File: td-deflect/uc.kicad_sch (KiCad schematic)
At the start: 20 parts, among them J4 Conn_ARM_JTAG_SWD_10, J6 Conn_01x06_Male, U12 LM1117-5.0, U2 STM32G474RETx, U23 TPS70933, U4 TPS70933, U8 INA181, X1 SG-8002CA

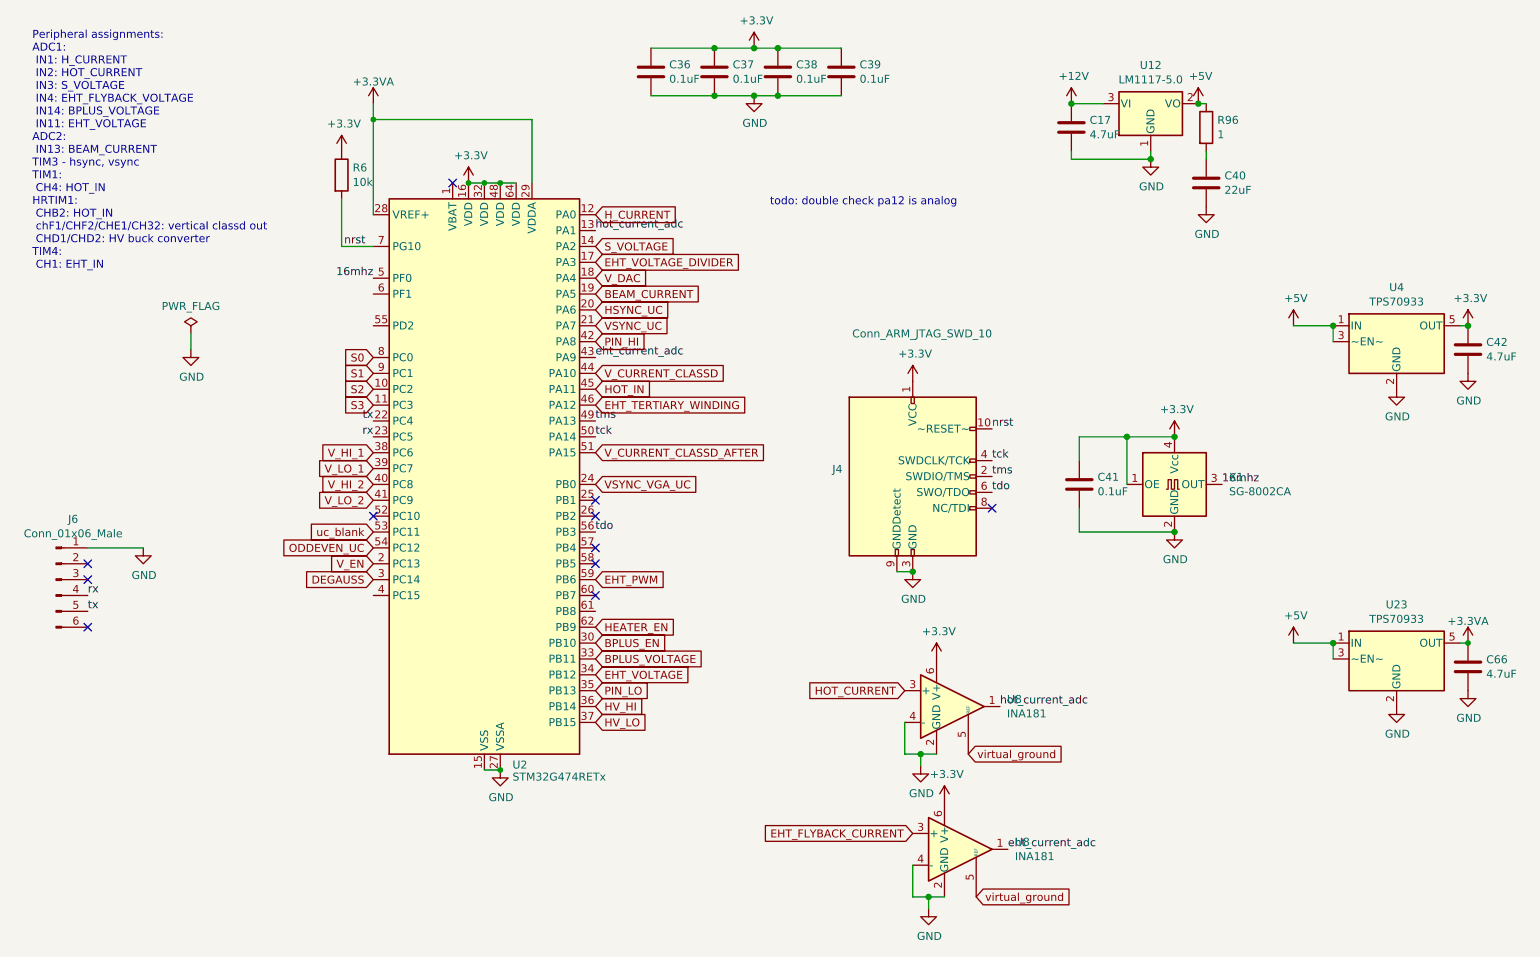
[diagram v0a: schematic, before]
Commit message: more updates
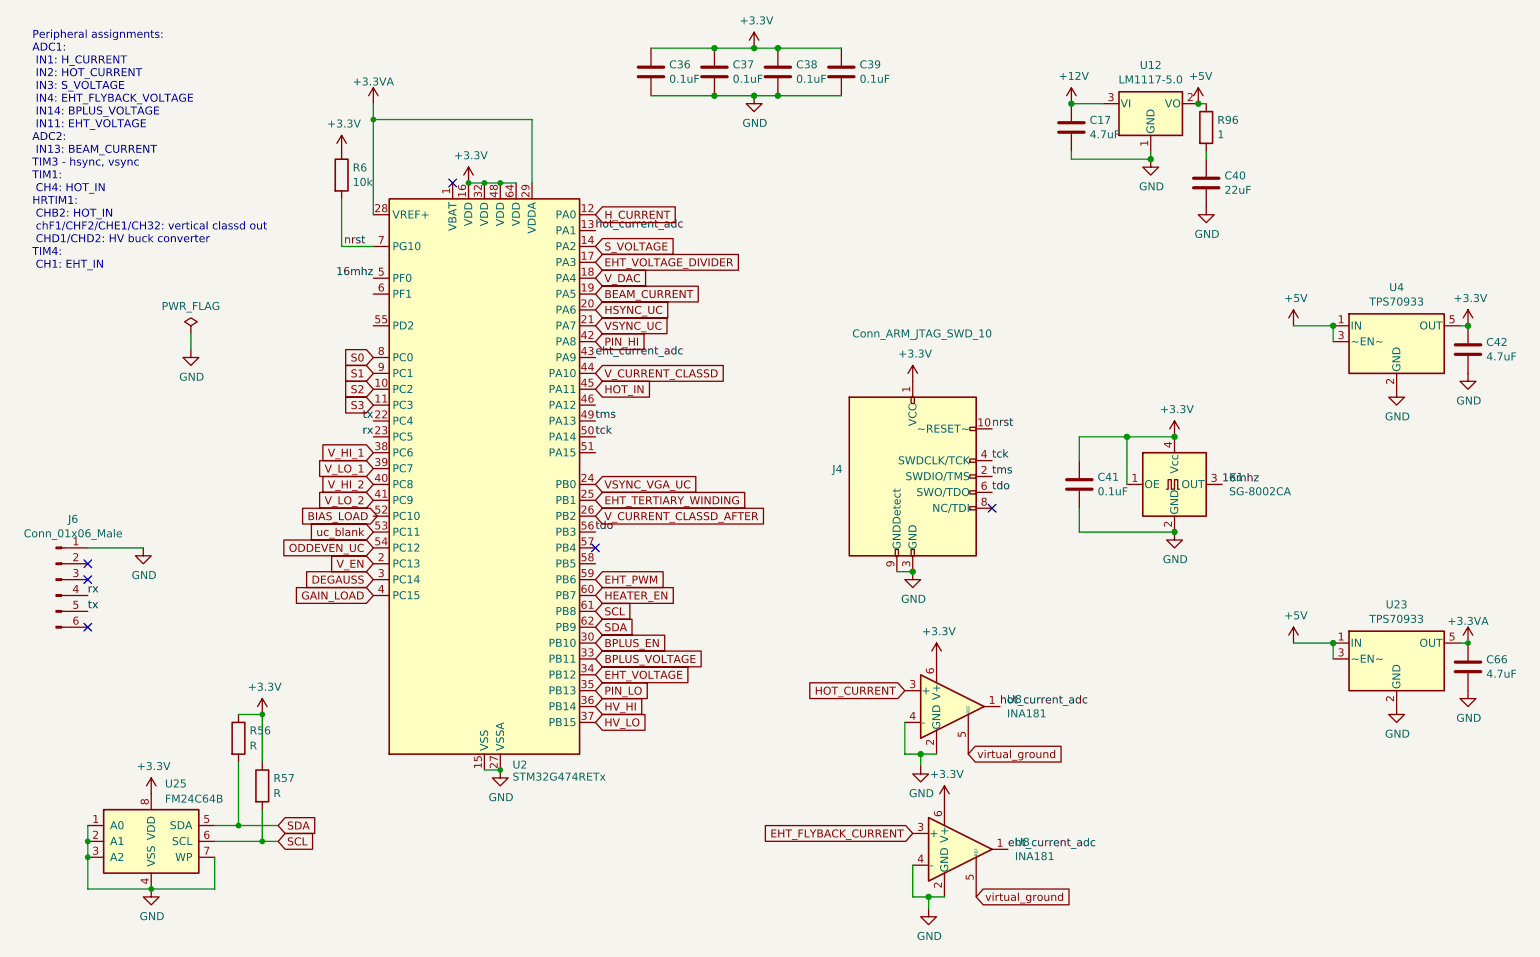
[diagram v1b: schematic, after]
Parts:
- added R56, R57: R, Resistor_SMD:R_0805_2012Metric_Pad1.15x1.40mm_HandSolder, symbol Device:R
- added U25: FM24C64B, Package_SO:SOIC-8_3.9x4.9mm_P1.27mm, symbol Memory_NVRAM:FM24C64B
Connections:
- net +3V3: now also R56.1, R57.1, U25.8 (VDD)
- net EHT_TERTIARY_WINDING: now also U2.25 (PB1); no longer U2.46 (PA12)
- net GND: now also U25.1 (A0), U25.2 (A1), U25.3 (A2), U25.4 (VSS), U25.7 (WP)
- net HEATER_EN: now also U2.60 (PB7); no longer U2.62 (PB9)
- net V_CURRENT_CLASSD_AFTER: now also U2.26 (PB2); no longer U2.51 (PA15)
- net GAIN_LOAD: now reaches U2.4 (PC15)
- net SCL: now reaches U2.61 (PB8)
- net SCL: now also R57.2, U25.6 (SCL)
- new net SDA: R56.2, U2.62 (PB9), U25.5 (SDA)
- no-connect marks 11 -> 6
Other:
- note removed: "todo: double check pa12 is analog"

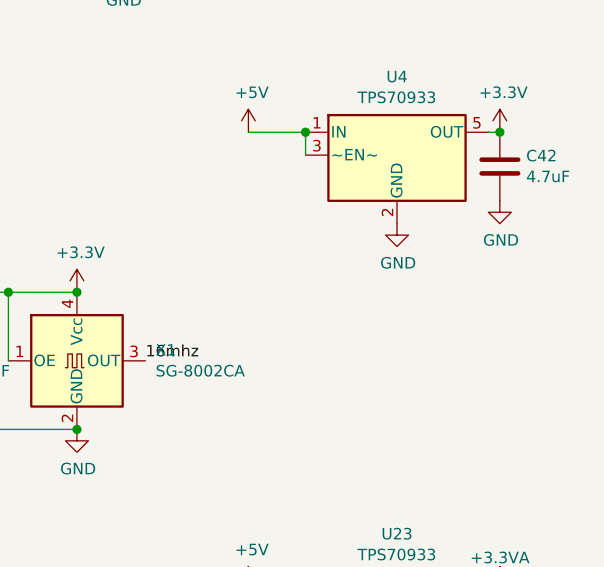
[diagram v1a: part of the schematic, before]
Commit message: small bugfix
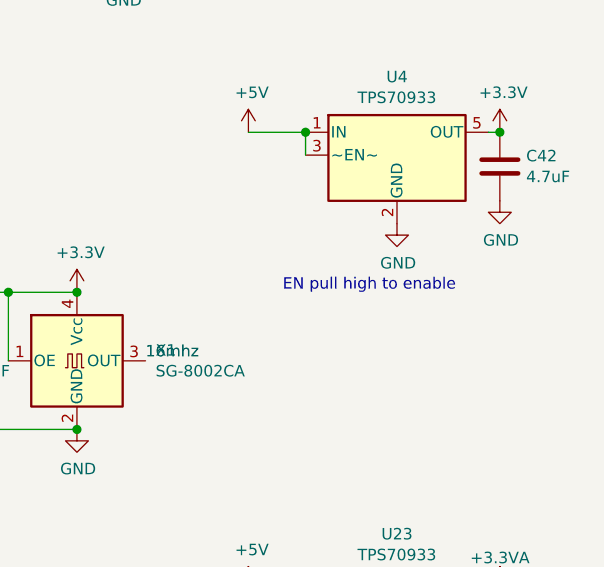
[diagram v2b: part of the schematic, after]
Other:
- note added: "EN pull high to enable"
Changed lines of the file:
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@@
+    (effects (font (size 1.27 1.27)) (justify left bottom))
+  )
+  (text "EN pull high to enable" (at 247.65 83.82 0)
     (effects (font (size 1.27 1.27)) (justify left bottom))
   )
